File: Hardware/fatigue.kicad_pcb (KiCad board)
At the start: 2 copper layers, 65 x 56 mm, 6 parts, among them J1 GPIO, U1 ADS1256IDBR

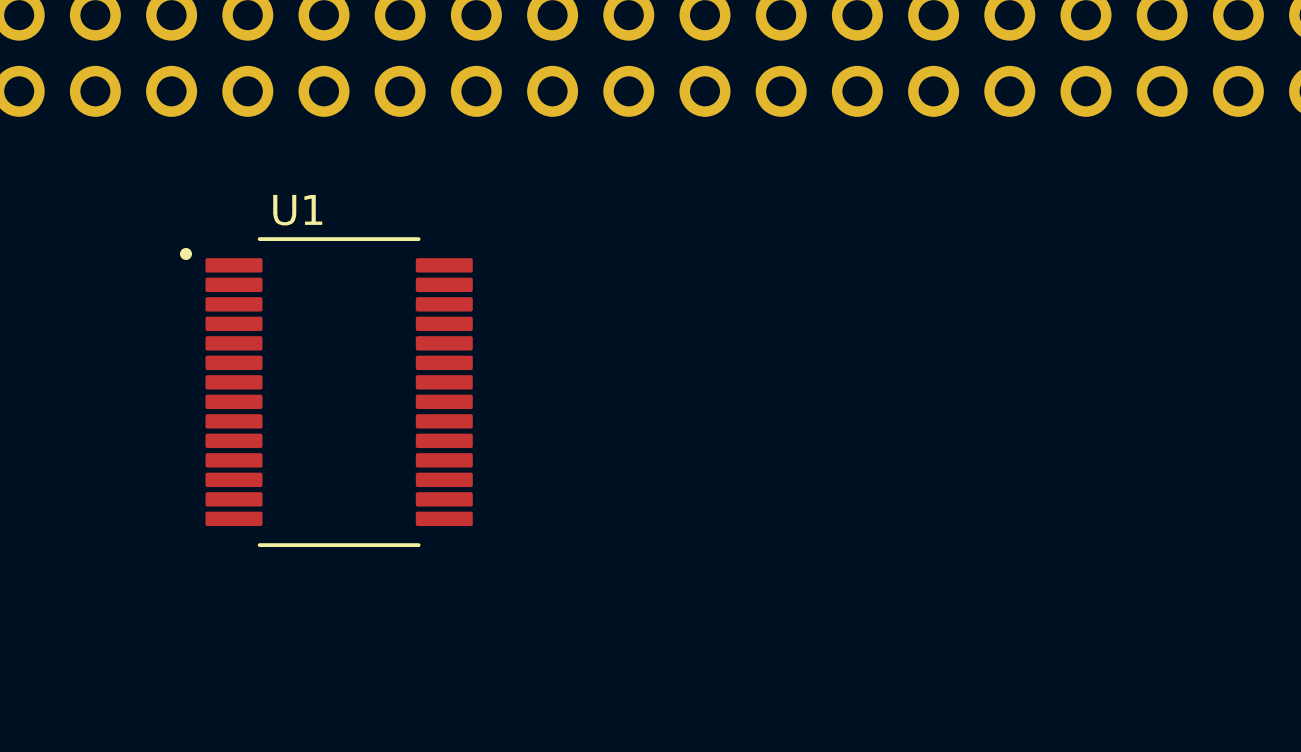
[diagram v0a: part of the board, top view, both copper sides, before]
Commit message: syncing this all up
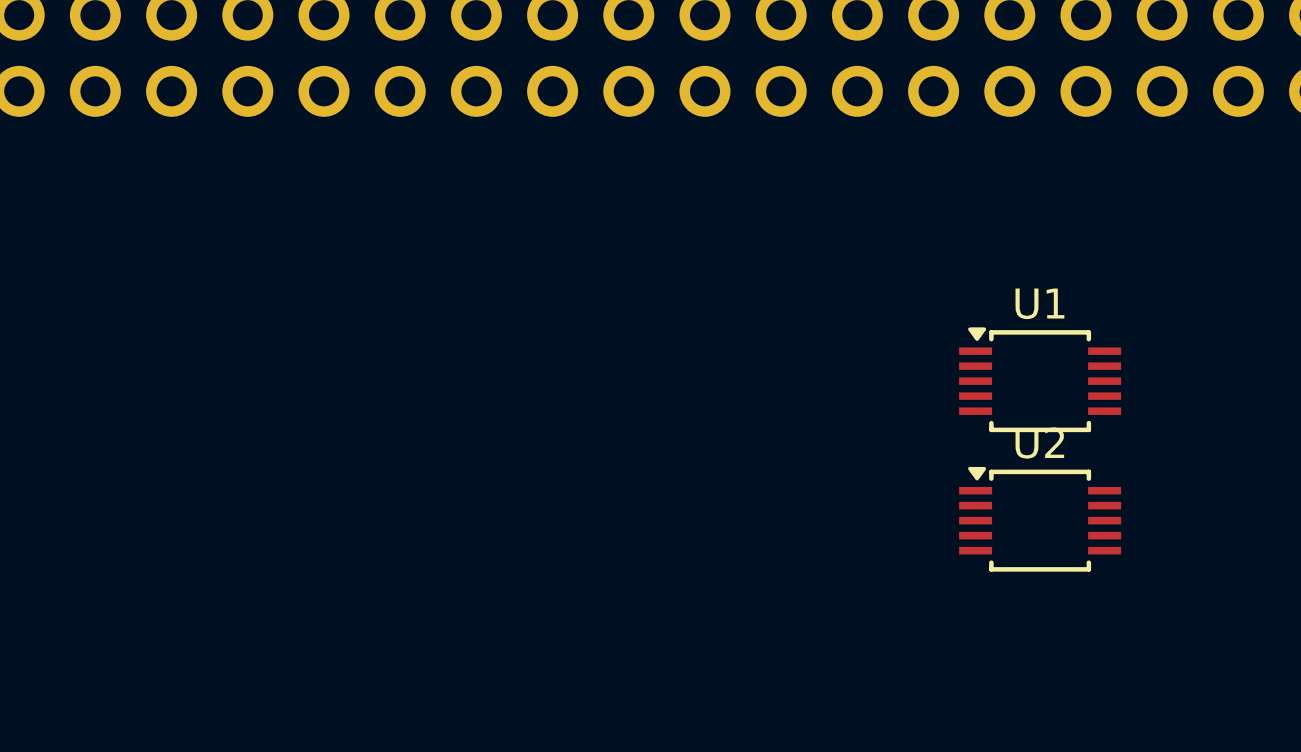
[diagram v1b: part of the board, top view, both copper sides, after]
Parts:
- added U2: ADS1115IDGS, Package_SO:TSSOP-10_3x3mm_P0.5mm, F.Cu at (147.5, 63.1)
- U1: value ADS1256IDBR -> ADS1115IDGS; footprint 1Personal:IC_ADC_ADS1256IDBR -> Package_SO:TSSOP-10_3x3mm_P0.5mm
- moved U1 23.4 mm to (147.5, 58.4)
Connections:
- J1 pad 2: +5V -> PI +5V
- J1 pad 4: +5V -> PI +5V
- U1 pad 10: unconnected-(U1-AIN4-Pad10) -> Net-(U1-SCL)
- U1 pad 2: GND -> Net-(U1-ALERT/RDY)
- U1 pad 3: unconnected-(U1-VREFN-Pad3) -> GND
- U1 pad 4: unconnected-(U1-VREFP-Pad4) -> Net-(U1-AIN0)
- U1 pad 5: unconnected-(U1-AINCOM-Pad5) -> GND
- U1 pad 6: unconnected-(U1-AIN0-Pad6) -> GND
- U1 pad 7: unconnected-(U1-AIN1-Pad7) -> GND
- U1 pad 8: unconnected-(U1-AIN2-Pad8) -> +5V
- U1 pad 9: unconnected-(U1-AIN3-Pad9) -> Net-(U1-SDA)
